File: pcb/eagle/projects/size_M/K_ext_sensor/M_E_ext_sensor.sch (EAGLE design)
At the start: 14 parts

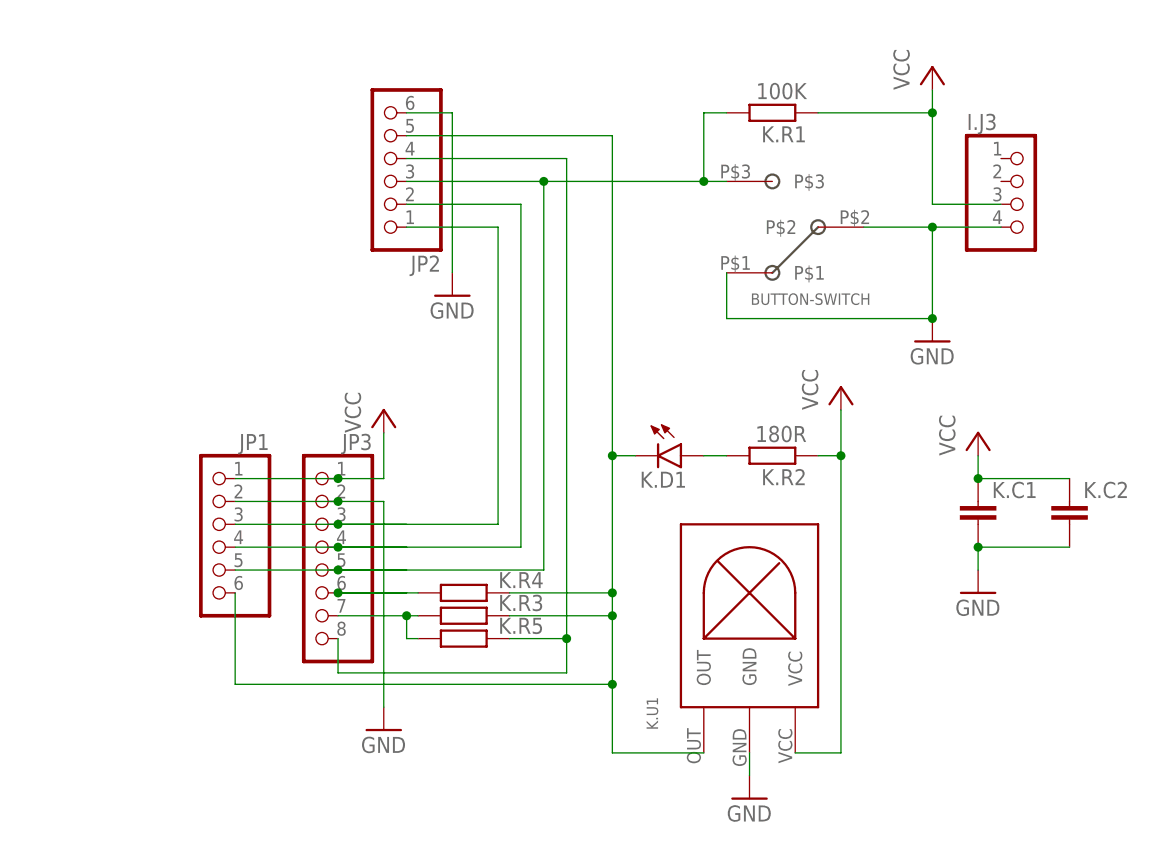
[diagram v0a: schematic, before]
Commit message: PCB v7 * 14 pin attiny is main adapter chip now. * changed adapter pin meaning (a1-a5, swapped RX-TX, VUSB replaced by A5, top most pin changed from GND to A4) * changed usb chip of main board
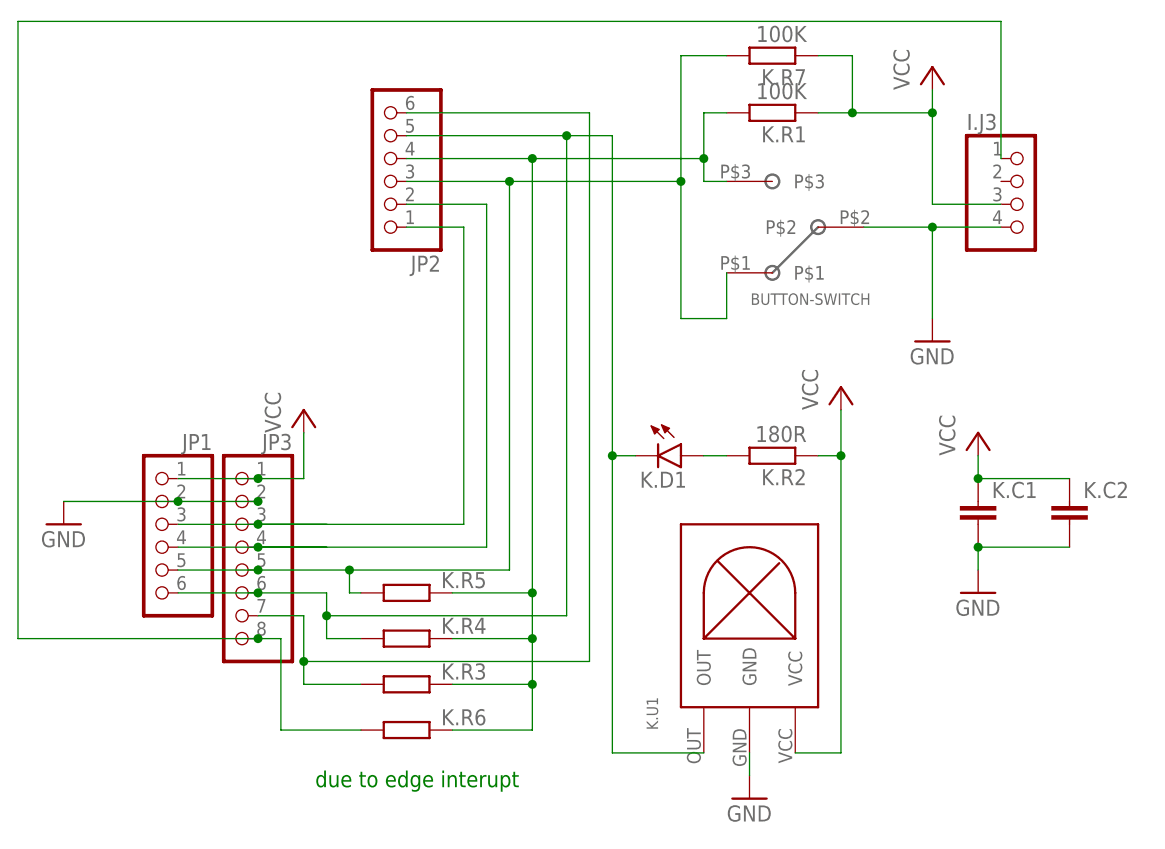
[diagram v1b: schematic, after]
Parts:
- added K.R6: 0R, rcl:R-EU_R0603
- added K.R7: 100K, rcl:R-EU_R0603
- K.D1: device led:LEDSML0603 -> led:LEDCHIP-LED0603
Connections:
- removed net N$1: JP1.5, JP2.3, JP3.5, K.R1.2, U$2.P$3
- removed net N$8: JP3.7, K.R3.2, K.R5.2
- new net N$10: JP1.6, JP2.5, JP3.6, K.D1.C, K.R4.2, K.U1.OUT
- new net N$9: I.J3.1, JP3.8, K.R6.2
- net GND: no longer JP2.6, U$2.P$1
- net N$2: now also JP2.4, K.R1.2, K.R5.1, K.R6.1, U$2.P$3; no longer JP1.6, JP2.5, K.D1.C, K.U1.OUT
- net N$3: now also JP1.5, JP2.3, JP3.5, K.R5.2, K.R7.2, U$2.P$1; no longer JP2.4, JP3.8, K.R5.1
- net N$7: now also JP2.6, JP3.7, K.R3.2; no longer JP3.6, K.R4.2
- net VCC: now also K.R7.1
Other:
- note added: "due to edge interupt"
- moved on the sheet: JP1, JP3, K.R3, K.R4, K.R5
